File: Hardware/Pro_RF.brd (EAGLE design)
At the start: 40.6 x 27.9 mm, 127 parts, among them J10 AVR_SPI_PROG_3X2TESTPOINTS, J12 JST, J7 PTH, J9 External On/Off, U1 MCP73831, U2 915MHz, U3 32U4, U6 3.3V, Y2 8MHz

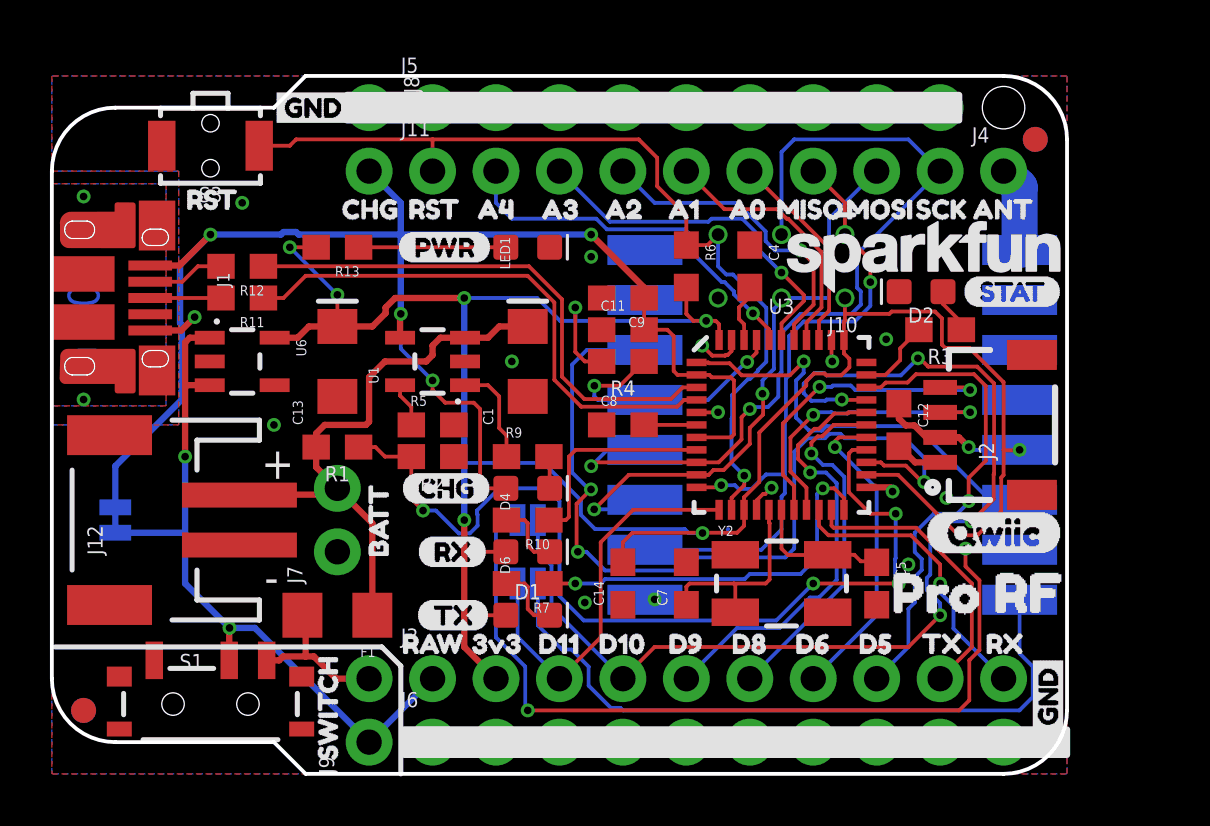
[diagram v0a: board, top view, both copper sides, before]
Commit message: Clean up
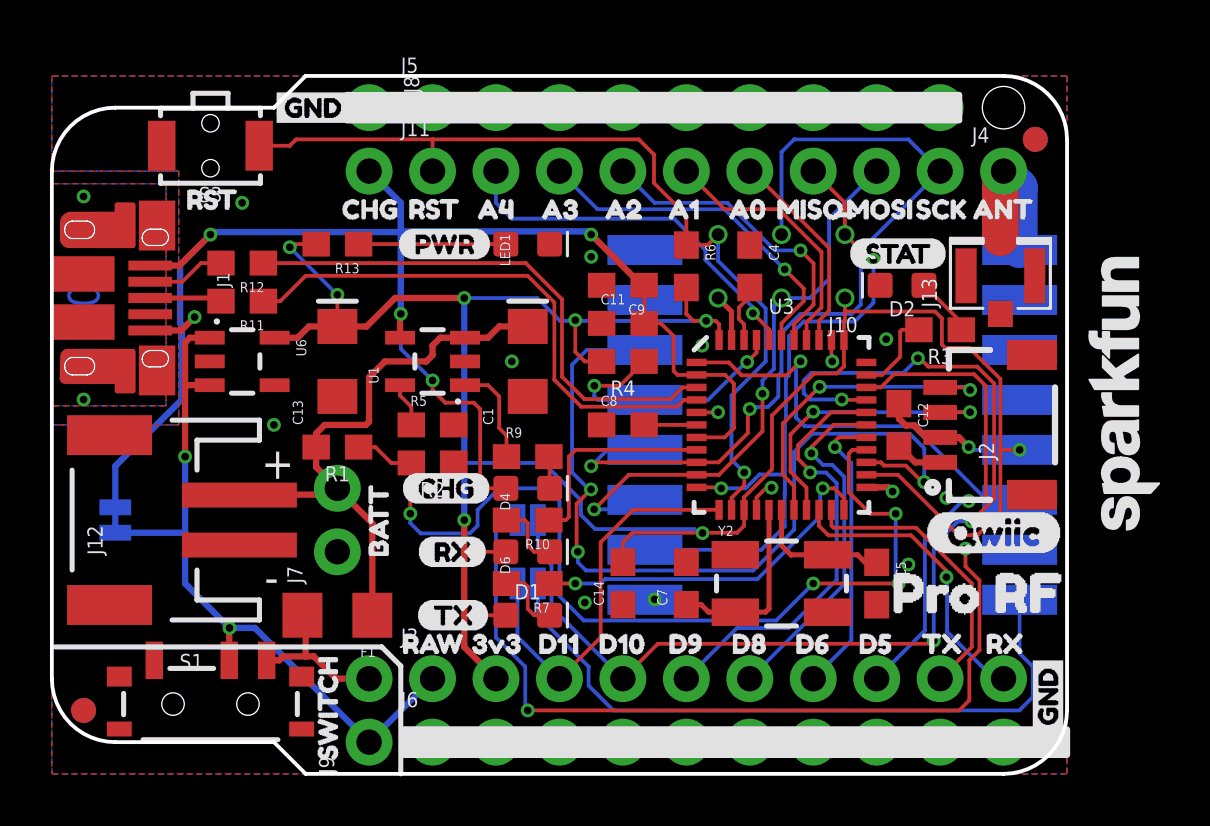
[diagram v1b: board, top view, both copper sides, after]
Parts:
- added J13: U.FL, SparkFun-Connectors:U.FL
- moved LOGO2 18.5 mm to (44.8, 9.27), turned to 90 degrees
- moved U$71 4.82 mm to (31.9, 20.8)
- moved D2 0.80 mm to (34.0, 19.6)
- moved C9 0.51 mm to (22.9, 19.6)
- moved R2 0.25 mm to (15.2, 12.4)
- moved C11 0.25 mm to (22.9, 18.0)
- moved R11 0.13 mm to (7.62, 18.9)
- moved LED1 0.13 mm to (19.1, 21.2)
- moved R12 0.13 mm to (7.62, 20.4)
- moved R13 0.13 mm to (11.4, 21.2)
- moved U$63 0.13 mm to (13.8, 21.2)
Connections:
- net ANT: now also J13.FEED
- net GND: now also J13.1, J13.2
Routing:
- net ANT: track 3.43 -> 6.14 mm
- net 3.3V: track 104.8 -> 103.2 mm
- net SHLD: track 0.21 -> 1.21 mm
- net TXLED: track 15.5 -> 14.6 mm
- net D6: track 12.6 -> 11.7 mm
- net N$6: track 8.15 -> 7.45 mm
- net N$3: track 1.85 -> 2.43 mm
- net MOSI: track 23.7 -> 23.2 mm
